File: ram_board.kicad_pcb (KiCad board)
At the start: 4 copper layers, 72.1 x 31.6 mm, 19 parts, among them J1 Conn_02x20_Odd_Even, J2 Conn_02x05_Odd_Even, SW1 SW_DIP_x04, U1 IS61LV5128AL-10TLI, U2 SST39VF040-70-4C-NHE, U3 74LVC04A

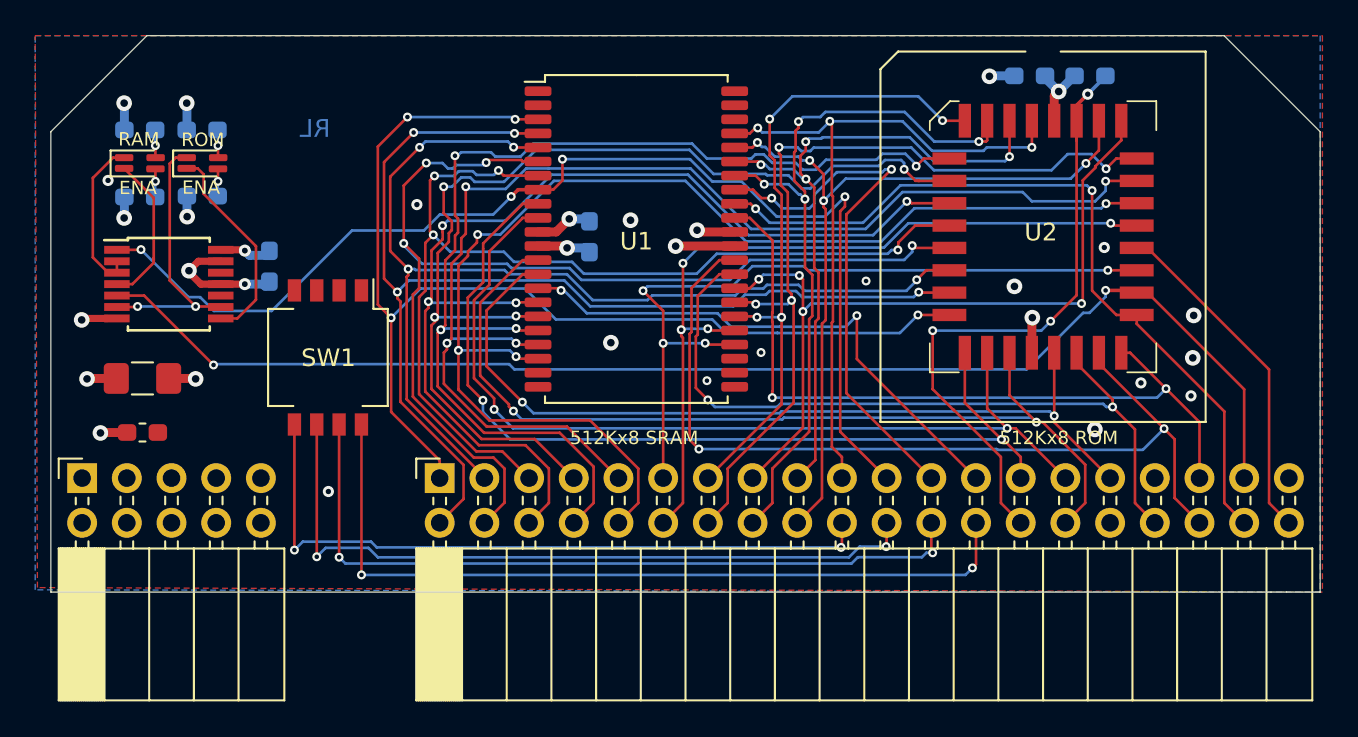
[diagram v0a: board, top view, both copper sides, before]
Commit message: redesign
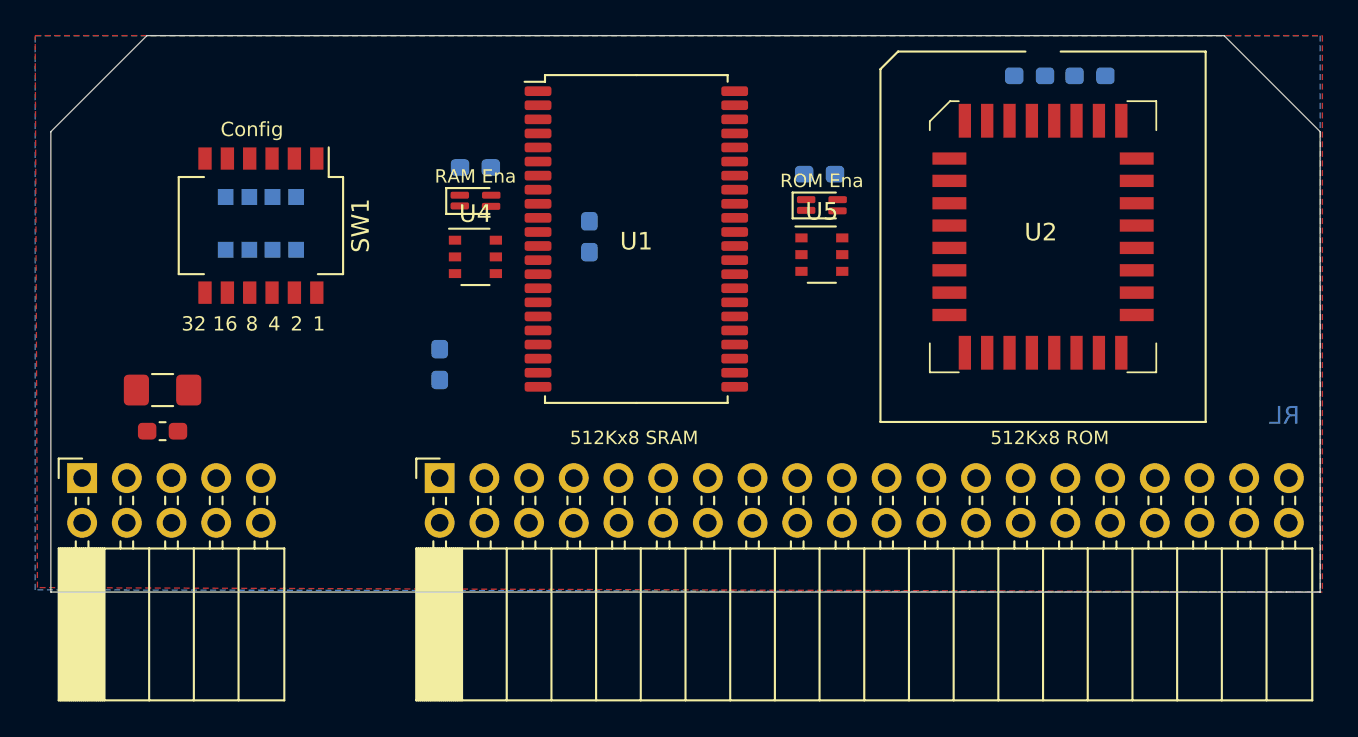
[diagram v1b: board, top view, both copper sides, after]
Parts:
- removed R4, R5, R6: 360R, Resistor_SMD:R_0603_1608Metric_Pad1.05x0.95mm_HandSolder
- removed U3: 74LVC04A, Package_SO:TSSOP-14_4.4x5mm_P0.65mm
- added R1: 360R, Resistor_SMD:R_0603_1608Metric_Pad1.05x0.95mm_HandSolder, B.Cu at (142.1, 80.0)
- added RN1: 1K, Resistor_SMD:R_Array_Convex_4x1206, B.Cu at (129.9, 83.2)
- added U4: 74LVC2G04, Package_SO:TSOP-6_1.65x3.05mm_P0.95mm, F.Cu at (142.1, 85.1)
- added U5: 74LVC2G04, Package_SO:TSOP-6_1.65x3.05mm_P0.95mm, F.Cu at (161.8, 85.0)
- J1: value Conn_02x20_Odd_Even -> Bus
- J2: value Conn_02x05_Odd_Even -> PWR
- R2: value 10K -> 1K
- SW1: value SW_DIP_x04 -> Config; footprint Button_Switch_SMD:SW_DIP_SPSTx04_Slide_KingTek_DSHP04TS_W7.62mm_P1.27mm -> Button_Switch_SMD:SW_DIP_SPSTx06_Slide_KingTek_DSHP06TS_W7.62mm_P1.27mm
- moved R3 38.7 mm to (161.7, 80.4), turned to 0 degrees
- moved D3 35.3 mm to (161.8, 82.2)
- moved D2 19.2 mm to (142.1, 81.9)
- moved C3 11.2 mm to (140.1, 91.2)
- moved SW1 8.41 mm to (129.9, 83.3)
- moved C4 1.32 mm to (124.3, 92.7), turned to 180 degrees
- moved C5 1.15 mm to (124.3, 95.0), turned to 180 degrees
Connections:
- D2 pad 3: Net-(D2-Pad3) -> Net-(D2-Pad1)
- D3 pad 3: Net-(D3-Pad3) -> Net-(D3-Pad1)
- J1 pad 1: /A0 -> GND
- J1 pad 10: /A9 -> /A1
- J1 pad 11: /A10 -> /A2
- J1 pad 12: /A11 -> /A3
- J1 pad 13: /A12 -> /A4
- J1 pad 14: /A13 -> /A5
- J1 pad 15: /A14 -> /A8
- J1 pad 16: /A15 -> /A7
- J1 pad 17: /A16 -> /A10
- J1 pad 18: /A17 -> /A9
- J1 pad 19: /A18 -> /A12
- J1 pad 2: /A1 -> /SW1_3
- J1 pad 20: /SW3 -> /A11
- J1 pad 21: /RAM_CE -> /A14
- J1 pad 22: /SW2 -> /A13
- J1 pad 23: /RAM_OE -> /A16
- J1 pad 24: /SW1 -> /A15
- J1 pad 25: /RAM_WE -> /A18
- J1 pad 26: /SW0 -> /A17
- J1 pad 27: /D0 -> /RAM_OE
- J1 pad 28: /ROM_WE -> /RAM_CE
- J1 pad 29: /D1 -> /D0
- J1 pad 3: /A2 -> (no net)
- J1 pad 30: /D2 -> /RAM_WE
- J1 pad 31: /D3 -> /D2
- J1 pad 32: GND -> /D1
- J1 pad 33: GND -> /D4
- J1 pad 34: /D4 -> /D3
- J1 pad 39: GND -> /ROM_WE
- J1 pad 4: /A3 -> /SW1_2
- J1 pad 5: /A4 -> (no net)
- J1 pad 6: /A5 -> /SW1_1
- J1 pad 7: /A6 -> (no net)
- J1 pad 8: /A7 -> /SW1_0
- J1 pad 9: /A8 -> /A0
- J2 pad 1: (no net) -> GND
- J2 pad 10: GND -> (no net)
- J2 pad 2: (no net) -> GND
- J2 pad 3: +3V3 -> GND
- J2 pad 4: +3V3 -> GND
- J2 pad 7: GND -> +3V3
- J2 pad 8: GND -> +3V3
- J2 pad 9: GND -> (no net)
- R3 pad 1: Net-(D2-Pad1) -> Net-(D3-Pad1)
- SW1 pad 5: /SW3 -> GND
- SW1 pad 6: /SW2 -> GND
- SW1 pad 7: /SW1 -> (no net)
- SW1 pad 8: /SW0 -> (no net)
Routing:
- net /ROM_CE: track 75.9 -> 0.00 mm, vias 2 -> 0
- net /A8: track 71.4 -> 0.00 mm, vias 4 -> 0
- net /A9: track 70.7 -> 0.00 mm, vias 4 -> 0
- net /RAM_CE: track 66.9 -> 0.00 mm, vias 4 -> 0
- net /A1: track 65.9 -> 0.00 mm, vias 4 -> 0
- net /A3: track 65.2 -> 0.00 mm, vias 4 -> 0
- net /A7: track 64.5 -> 0.00 mm, vias 4 -> 0
- net /A0: track 64.0 -> 0.00 mm, vias 4 -> 0
- net /A2: track 61.3 -> 0.00 mm, vias 4 -> 0
- net /A5: track 61.2 -> 0.00 mm, vias 4 -> 0
- net /A6: track 60.6 -> 0.00 mm, vias 4 -> 0
- net /A4: track 59.1 -> 0.00 mm, vias 4 -> 0
- net /D2: track 54.0 -> 0.00 mm, vias 2 -> 0
- net /D0: track 53.6 -> 0.00 mm, vias 2 -> 0
- net /D1: track 52.2 -> 0.00 mm, vias 2 -> 0
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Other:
- board text added: "1"
- board text added: "16"
- board text added: "2"
- board text added: "32"
- board text added: "4"
- board text added: "8"
- board text added: "Config"
- board text added: "MAX V RAM/ROM Extension v1.0 © 2019 by Hyiger Designs Made for: DeltaBrd http://ilchev.net/deltabrd"
- board text added: "RAM Ena"
- board text added: "ROM Ena"
- board text removed: "DeltaBrd RAM/ROM Extension v1.0 © 2019 by Hyiger Designs"
- board text removed: "ENA"
- board text removed: "RAM"
- board text removed: "ROM"
